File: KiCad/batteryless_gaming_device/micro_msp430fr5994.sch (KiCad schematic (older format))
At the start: 17 parts, among them J400 GPIO_breakout, J401 Multiplayer_Connector, J402 Program_Header, SW400 FSMSM, U400 MSP430FR5994, U401 SN74HCS32, Y400 ECS-.327-12.5-34R-C-TR

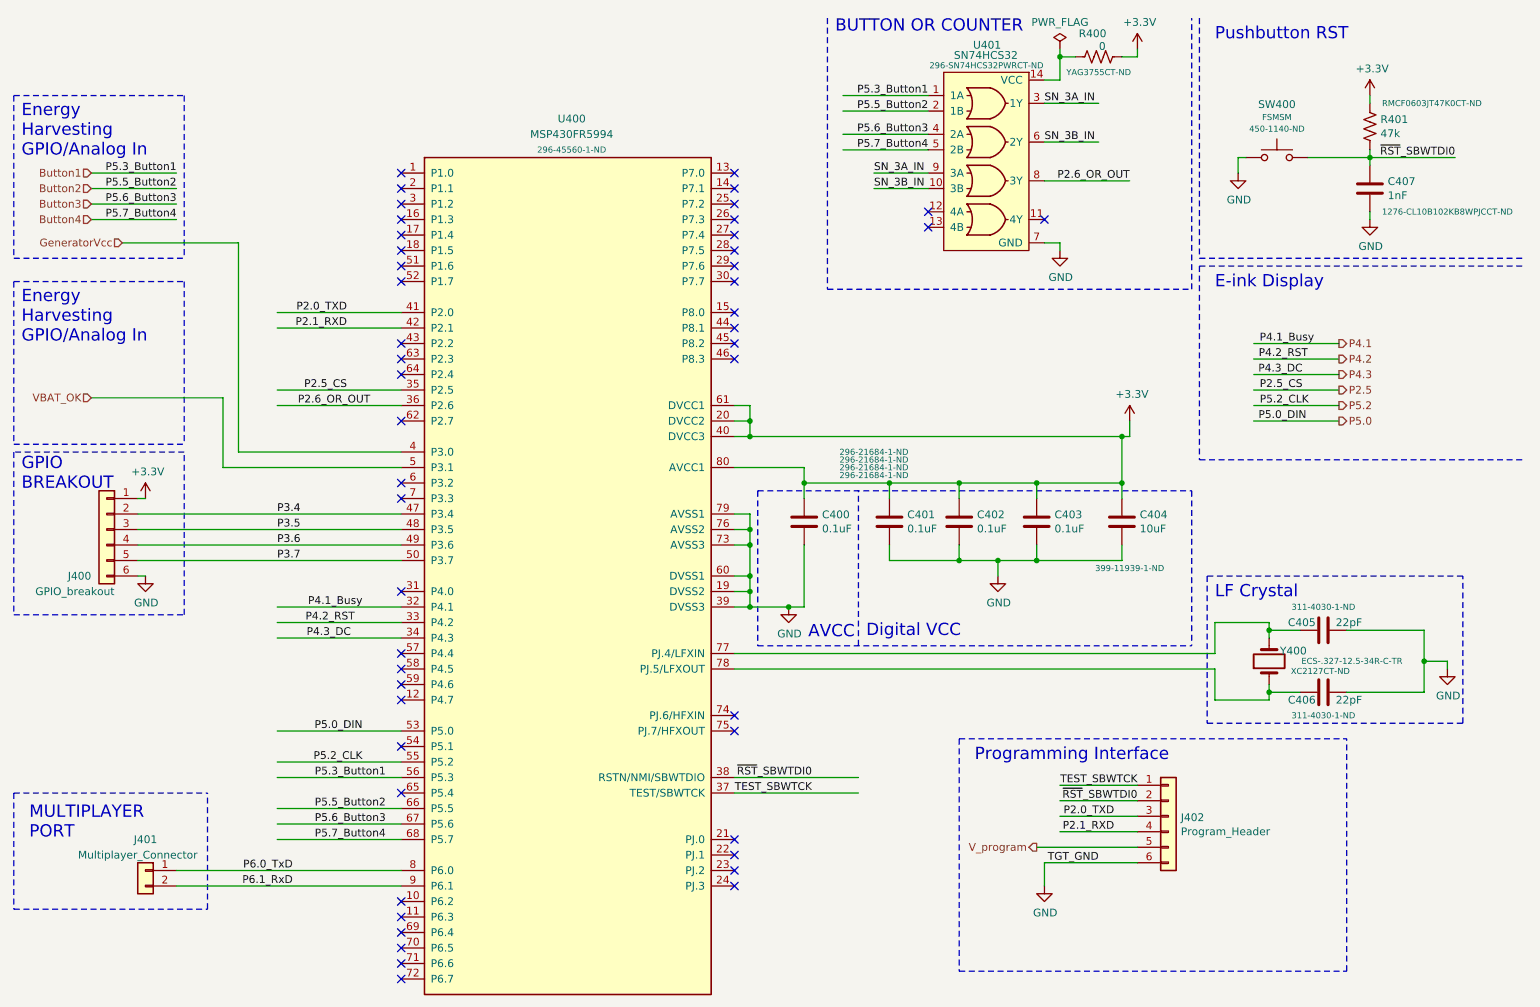
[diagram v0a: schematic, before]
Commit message: oh ya
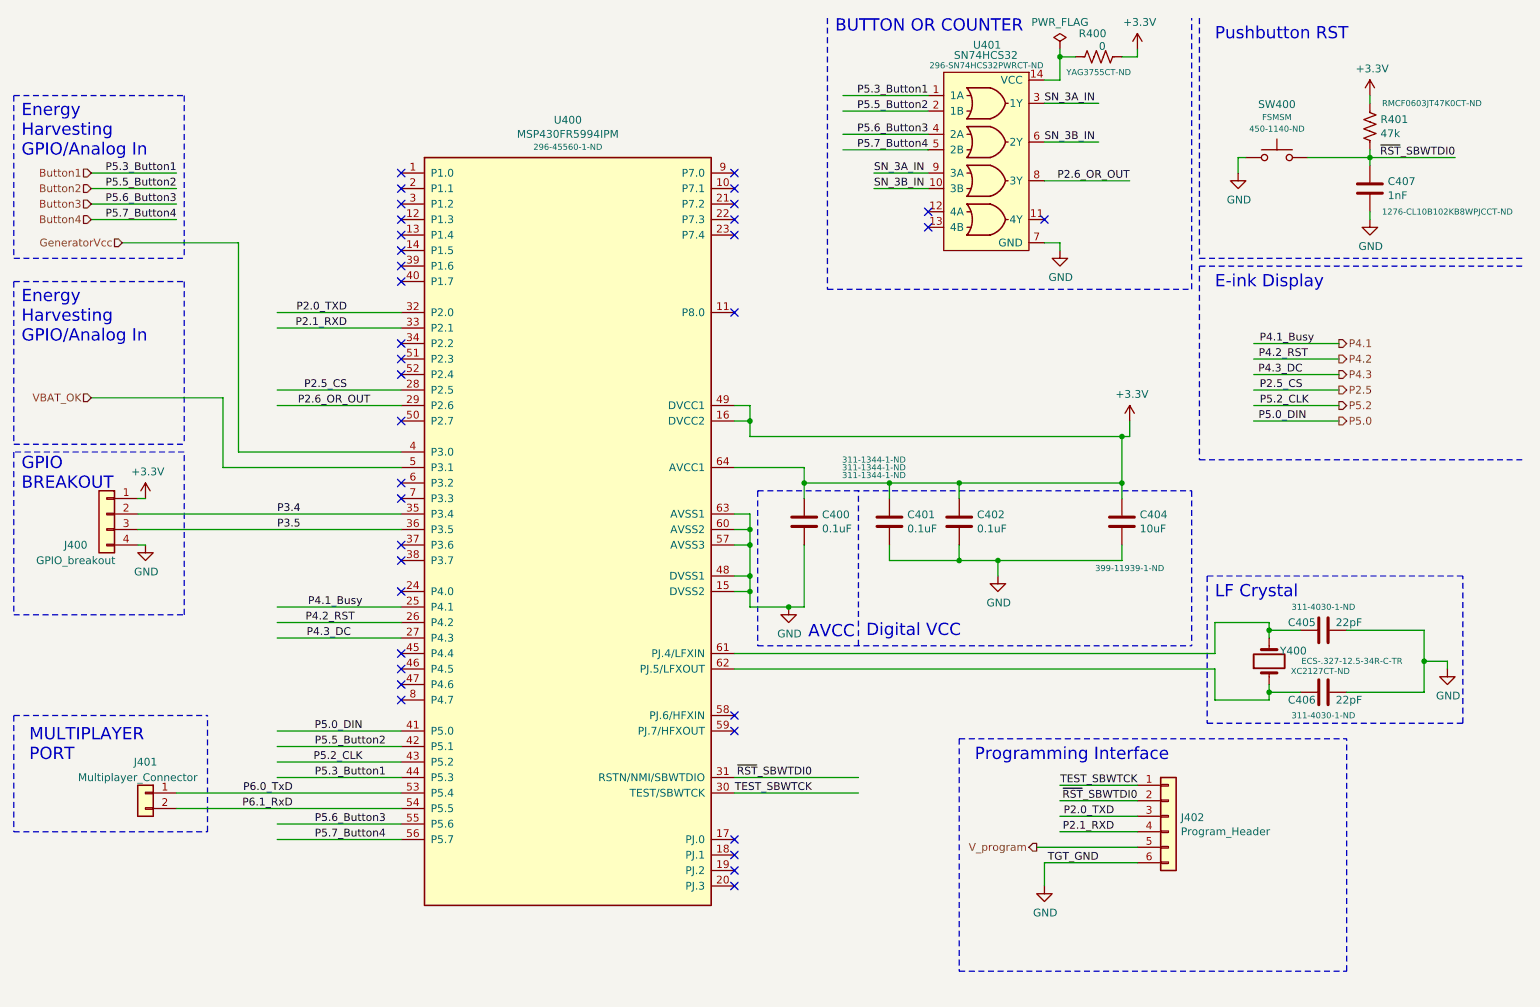
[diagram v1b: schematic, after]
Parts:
- removed C403: 0.1uF, Capacitor_SMD:C_0603_1608Metric_Pad1.08x0.95mm_HandSolder, symbol Device:C
- removed J400: GPIO_breakout, Connector_PinHeader_2.54mm:PinHeader_1x06_P2.54mm_Vertical, symbol Connector_Generic:Conn_01x06
- removed U400: MSP430FR5994, Package_QFP:LQFP-64_10x10mm_P0.5mm, symbol batteryless_gaming_device-rescue:MSP430FR5994
- added J400: GPIO_breakout, Connector_PinHeader_2.54mm:PinHeader_1x04_P2.54mm_Vertical, symbol Connector_Generic:Conn_01x04
- added U400: MSP430FR5994IPM, Package_QFP:LQFP-64_10x10mm_P0.5mm, symbol batteryless_gaming_device-rescue:MSP430FR5994IPM
- C400, C401, C402: Digikey PN 296-21684-1-ND -> 311-1344-1-ND
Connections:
- net labels removed: P3.6, P3.7
- wire segments 132 -> 124
- no-connect marks 48 -> 36
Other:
- moved on the sheet: J401
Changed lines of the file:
@@
 $EndDescr
-$Comp
-L batteryless_gaming_device-rescue:MSP430FR5994 U?
-U 1 1 6192B25C
-P 4300 1400
-AR Path="/6192B25C" Ref="U?"  Part="1"
-AR Path="/61926AE2/6192B25C" Ref="U400"  Part="1"
-F 0 "U400" H 4350 1650 50  0000 C CNN
-F 1 "MSP430FR5994" H 4350 1550 50  0000 C CNN
-F 2 "Package_QFP:LQFP-64_10x10mm_P0.5mm" V 3400 1200 354 0001 C CNN
-F 3 "" V 3400 1200 354 0001 C CNN
-F 4 "296-45560-1-ND" H 4350 1450 39  0000 C CNN "Digikey PN"
-	1    4300 1400
-	1    0    0    -1
-$EndComp
 $Comp
 L Device:C C400
@@
 F 2 "Capacitor_SMD:C_0603_1608Metric_Pad1.08x0.95mm_HandSolder" H 5888 3600 50  0001 C CNN
 F 3 "~" H 5850 3750 50  0001 C CNN
-F 4 "296-21684-1-ND" H 6300 4050 39  0000 C CNN "Digikey PN"
+F 4 "311-1344-1-ND" H 6300 4050 39  0000 C CNN "Digikey PN"
 	1    5850 3750
 	1    0    0    -1
@@
 Wire Wire Line
 	5500 4200 5500 4300
-Wire Wire Line
-	5500 4300 5400 4300
 Connection ~ 5500 4200
 $Comp
@@
 Wire Wire Line
 	5500 4300 5750 4300
-Connection ~ 5500 4300
 Wire Wire Line
 	5750 4300 5850 4300
@@
 Connection ~ 5750 4300
 Wire Wire Line
-	5500 3200 5400 3200
-Wire Wire Line
 	5500 3200 5500 3100
 Wire Wire Line
@@
 	5500 3000 5400 3000
 Connection ~ 5500 3100
-Connection ~ 5500 3200
 $Comp
 L power:+3.3V #PWR0406
@@
 NoConn ~ 5400 6100
 NoConn ~ 5400 1900
-NoConn ~ 5400 2000
-NoConn ~ 5400 2100
-NoConn ~ 5400 2200
 NoConn ~ 3250 3100
 NoConn ~ 3250 2700
@@
 NoConn ~ 3250 4700
 NoConn ~ 3250 4800
-NoConn ~ 3250 5500
-NoConn ~ 3250 6400
-NoConn ~ 3250 6500
-NoConn ~ 3250 6600
-NoConn ~ 3250 6700
 Text Label 5900 5500 2    50   ~ 0
 TEST_SBWTCK
@@
 Wire Notes Line
 	8350 3550 8350 4550
-Wire Wire Line
-	7100 4000 7350 4000
 Connection ~ 7100 4000
 Wire Wire Line
 	7100 4100 7100 4000
-Connection ~ 7350 4000
 Wire Wire Line
 	7900 4000 7900 3900
-Wire Wire Line
-	7350 4000 7900 4000
 Connection ~ 6850 4000
-Wire Wire Line
-	7350 4000 7350 3900
 Wire Wire Line
 	6850 4000 7100 4000
@@
 Wire Wire Line
 	6850 3500 6400 3500
-Connection ~ 7350 3500
 Wire Wire Line
 	6850 3500 6850 3600
-Wire Wire Line
-	7350 3500 6850 3500
 Wire Wire Line
 	7900 3500 7900 3600
 Connection ~ 7900 3500
 Wire Wire Line
-	7350 3500 7350 3600
-Wire Wire Line
-	7900 3500 7350 3500
-Wire Wire Line
 	7900 3200 7900 3500
-$Comp
-L Device:C C403
-U 1 1 619313AD
-P 7350 3750
-F 0 "C403" H 7465 3796 50  0000 L CNN
-F 1 "0.1uF" H 7465 3705 50  0000 L CNN
-F 2 "Capacitor_SMD:C_0603_1608Metric_Pad1.08x0.95mm_HandSolder" H 7388 3600 50  0001 C CNN
-F 3 "~" H 7350 3750 50  0001 C CNN
-F 4 "296-21684-1-ND" H 6300 4200 39  0000 C CNN "Digikey PN"
-	1    7350 3750
-	1    0    0    -1
-$EndComp
 $Comp
 L Device:C C402
@@
 F 2 "Capacitor_SMD:C_0603_1608Metric_Pad1.08x0.95mm_HandSolder" H 6888 3600 50  0001 C CNN
 F 3 "~" H 6850 3750 50  0001 C CNN
-F 4 "296-21684-1-ND" H 6300 4150 39  0000 C CNN "Digikey PN"
+F 4 "311-1344-1-ND" H 6300 4150 39  0000 C CNN "Digikey PN"
 	1    6850 3750
 	1    0    0    -1
@@
 F 2 "Capacitor_SMD:C_0603_1608Metric_Pad1.08x0.95mm_HandSolder" H 6438 3600 50  0001 C CNN
 F 3 "~" H 6400 3750 50  0001 C CNN
-F 4 "296-21684-1-ND" H 6300 4100 39  0000 C CNN "Digikey PN"
+F 4 "311-1344-1-ND" H 6300 4100 39  0000 C CNN "Digikey PN"
 	1    6400 3750
 	1    0    0    -1
@@
 	3250 5400 2450 5400
 Wire Wire Line
-	3250 5600 2450 5600
+	3250 5200 2450 5200
 Wire Wire Line
 	3250 5700 2450 5700
@@
 Text Label 3150 5400 2    50   ~ 0
 P5.3_Button1
-Text Label 3150 5600 2    50   ~ 0
+Text Label 3150 5200 2    50   ~ 0
 P5.5_Button2
 Text Label 3150 5700 2    50   ~ 0
@@
 NoConn ~ 7400 1800
 Wire Wire Line
-	3250 6000 1800 6000
-Wire Wire Line
-	3250 6100 1800 6100
+	3250 5500 1800 5500
+Wire Wire Line
+	3250 5600 1800 5600
 $Comp
 L Connector_Generic:Conn_01x02 J401
 U 1 1 61A8E8B4
-P 1600 6000
-F 0 "J401" H 1600 6200 50  0000 C CNN
-F 1 "Multiplayer_Connector" H 1650 6100 50  0000 C CNN
-F 2 "Connector_PinHeader_2.54mm:PinHeader_1x02_P2.54mm_Horizontal" H 1600 6000 50  0001 C CNN
-F 3 "~" H 1600 6000 50  0001 C CNN
-	1    1600 6000
+P 1600 5500
+F 0 "J401" H 1600 5700 50  0000 C CNN
+F 1 "Multiplayer_Connector" H 1650 5600 50  0000 C CNN
+F 2 "Connector_PinHeader_2.54mm:PinHeader_1x02_P2.54mm_Horizontal" H 1600 5500 50  0001 C CNN
+F 3 "~" H 1600 5500 50  0001 C CNN
+	1    1600 5500
 	-1   0    0    -1
 $EndComp
-Text Label 2550 6000 2    50   ~ 0
+Text Label 2550 5500 2    50   ~ 0
 P6.0_TxD
-Text Label 2550 6100 2    50   ~ 0
+Text Label 2550 5600 2    50   ~ 0
 P6.1_RxD
 Wire Notes Line
-	750  5500 750  6250
-Wire Notes Line
-	750  6250 2000 6250
-Wire Notes Line
-	2000 6250 2000 5500
-Wire Notes Line
-	750  5500 2000 5500
-Text Notes 850  5800 0    79   ~ 0
+	750  5000 750  5750
+Wire Notes Line
+	750  5750 2000 5750
+Wire Notes Line
+	2000 5750 2000 5000
+Wire Notes Line
+	750  5000 2000 5000
+Text Notes 850  5300 0    79   ~ 0
 MULTIPLAYER\nPORT
-$Comp
-L Connector_Generic:Conn_01x06 J400
-U 1 1 61AD4142
-P 1350 3800
-F 0 "J400" H 1450 3500 50  0000 L CNN
-F 1 "GPIO_breakout" H 1300 3400 50  0000 L CNN
-F 2 "Connector_PinHeader_2.54mm:PinHeader_1x06_P2.54mm_Vertical" H 1350 3800 50  0001 C CNN
-F 3 "~" H 1350 3800 50  0001 C CNN
-	1    1350 3800
-	-1   0    0    -1
-$EndComp
 Wire Wire Line
 	1550 3700 3250 3700
@@
 L power:GND #PWR0401
 U 1 1 61AFF4BE
-P 1600 4100
-F 0 "#PWR0401" H 1600 3850 50  0001 C CNN
-F 1 "GND" H 1605 3927 50  0000 C CNN
-F 2 "" H 1600 4100 50  0001 C CNN
-F 3 "" H 1600 4100 50  0001 C CNN
-	1    1600 4100
-	1    0    0    -1
-$EndComp
-Wire Wire Line
-	1550 4100 1600 4100
-Wire Wire Line
-	1550 3900 3250 3900
+P 1600 3900
+F 0 "#PWR0401" H 1600 3650 50  0001 C CNN
+F 1 "GND" H 1605 3727 50  0000 C CNN
+F 2 "" H 1600 3900 50  0001 C CNN
+F 3 "" H 1600 3900 50  0001 C CNN
+	1    1600 3900
+	1    0    0    -1
+$EndComp
+Wire Wire Line
+	1550 3900 1600 3900
 Wire Wire Line
 	1550 3600 1600 3600
@@
 Text Label 2600 3800 2    50   ~ 0
 P3.5
-Text Label 2600 3900 2    50   ~ 0
-P3.6
-Wire Wire Line
-	1550 4000 3250 4000
-Text Label 2600 4000 2    50   ~ 0
-P3.7
 Wire Notes Line
 	750  3300 750  4350
@@
 Text Notes 800  3550 0    79   ~ 0
 GPIO\nBREAKOUT
-NoConn ~ 3250 6200
-NoConn ~ 3250 6300
-NoConn ~ 3250 5200
 NoConn ~ 3250 4900
 NoConn ~ 3250 4600
@@
 NoConn ~ 5400 1800
 NoConn ~ 5400 2400
-NoConn ~ 5400 2500
-NoConn ~ 5400 2600
-NoConn ~ 5400 2700
 NoConn ~ 5400 5000
 NoConn ~ 5400 5100
@@
 	7500 700  7500 750
 Connection ~ 7500 750
+$Comp
+L batteryless_gaming_device-rescue:MSP430FR5994IPM U400
+U 1 1 61A050A0
+P 4300 1400
+F 0 "U400" H 4325 1642 50  0000 C CNN
+F 1 "MSP430FR5994IPM" H 4325 1551 50  0000 C CNN
+F 2 "Package_QFP:LQFP-64_10x10mm_P0.5mm" H 4325 1650 50  0001 C CNN
+F 3 "" H 4325 1650 50  0001 C CNN
+F 4 "296-45560-1-ND" H 4325 1468 39  0000 C CNN "Digikey PN"
+	1    4300 1400
+	1    0    0    -1
+$EndComp
+Wire Wire Line
+	7100 4000 7900 4000
+Wire Wire Line
+	6850 3500 7900 3500
+$Comp
+L Connector_Generic:Conn_01x04 J400
+U 1 1 61AD24EA
+P 1350 3700
+F 0 "J400" H 1550 3500 50  0000 C CNN
+F 1 "GPIO_breakout" H 1550 3400 50  0000 C CNN
+F 2 "Connector_PinHeader_2.54mm:PinHeader_1x04_P2.54mm_Vertical" H 1350 3700 50  0001 C CNN
+F 3 "~" H 1350 3700 50  0001 C CNN
+	1    1350 3700
+	-1   0    0    -1
+$EndComp
+NoConn ~ 3250 3900
+NoConn ~ 3250 4000
 $EndSCHEMATC
